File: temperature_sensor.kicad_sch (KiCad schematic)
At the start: 3 parts, among them U3 XIAO-SAMD21-SMD, U5 TMP37FT9Z

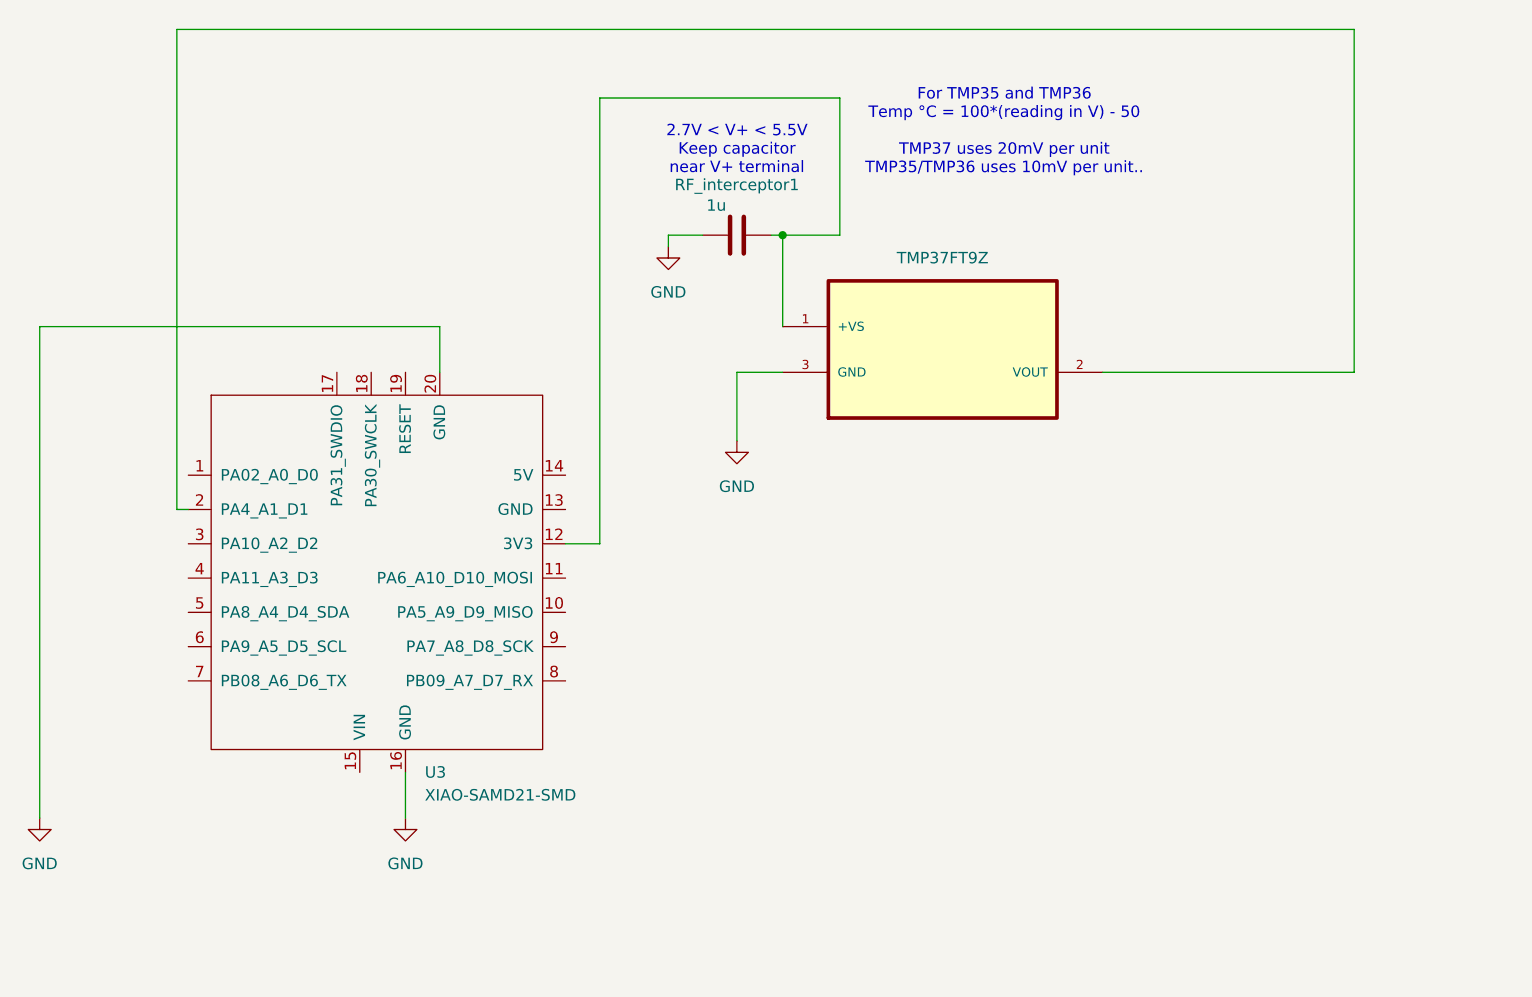
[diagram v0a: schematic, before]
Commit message: ok yeah no
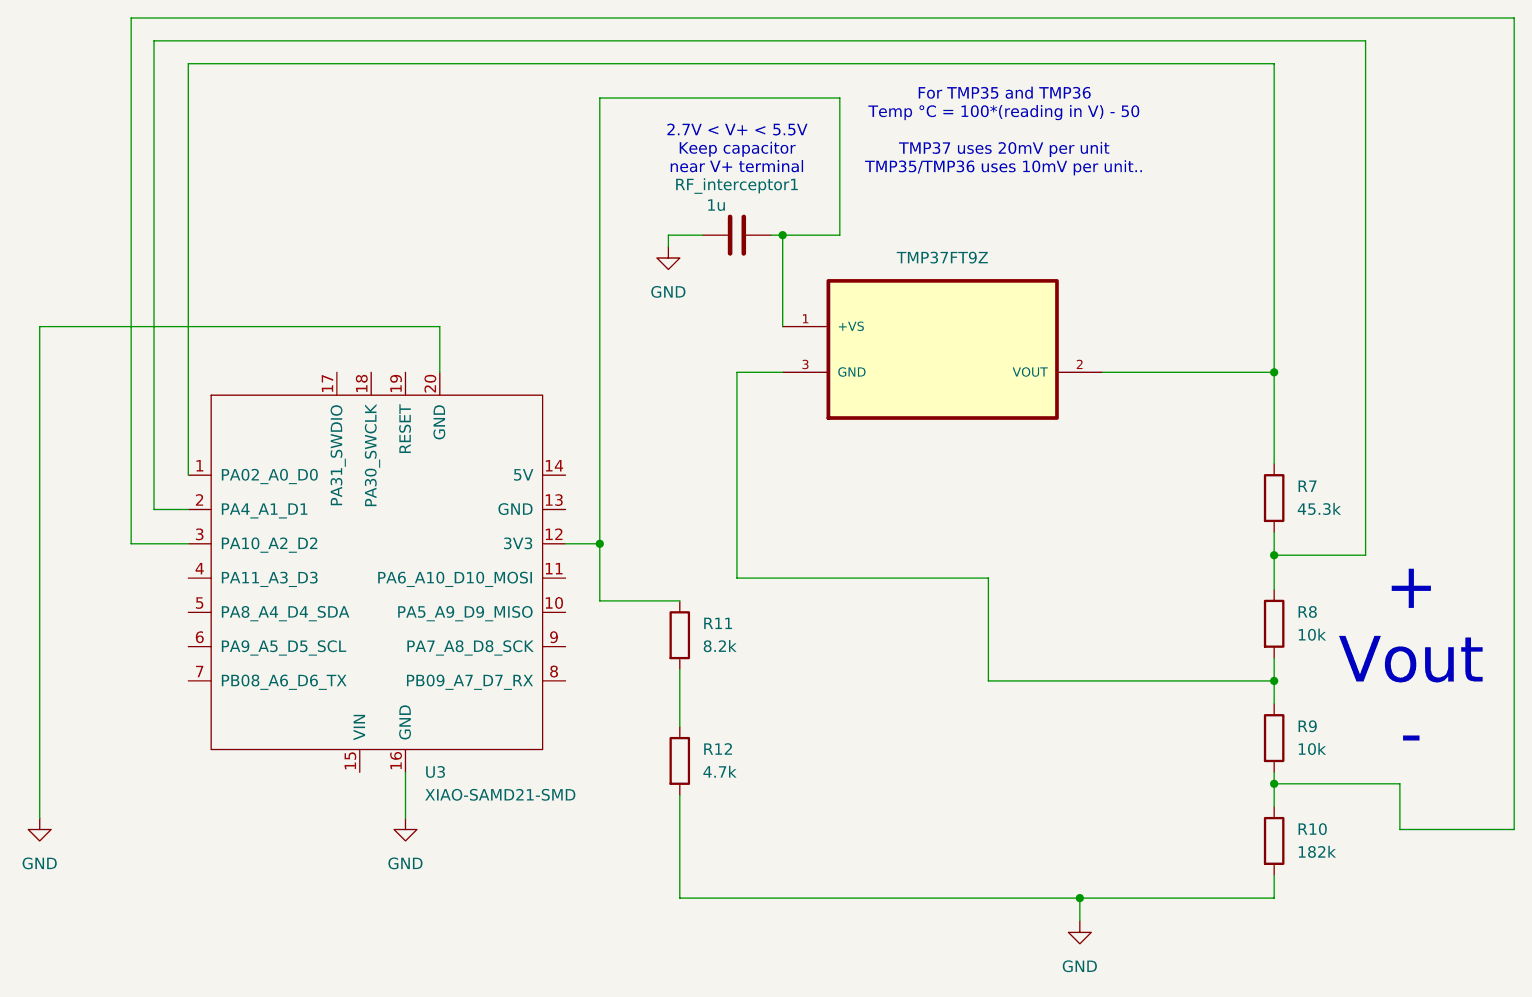
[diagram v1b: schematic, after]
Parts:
- added R10: 182k, Resistor_SMD:R_1210_3225Metric_Pad1.30x2.65mm_HandSolder, symbol Device:R
- added R11: 8.2k, R_1210_3225Metric_Pad1.30x2.65mm_HandSolder, symbol Device:R
- added R12: 4.7k, R_1210_3225Metric_Pad1.30x2.65mm_HandSolder, symbol Device:R
- added R7: 45.3k, R_1210_3225Metric_Pad1.30x2.65mm_HandSolder, symbol Device:R
- added R8, R9: 10k, R_1210_3225Metric_Pad1.30x2.65mm_HandSolder, symbol Device:R
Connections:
- net GND: now also R10.2, R12.2; no longer U5.3 (GND)
- net at RF_interceptor1.2, U3.12 (3V3), U5.1 (+VS): now also R11.1
- net at U5.2 (VOUT): now also U3.1 (PA02_A0_D0), R7.1; no longer U3.2 (PA4_A1_D1)
- net at U3.3 (PA10_A2_D2): now also R10.1, R9.2
- new net: R11.2, R12.1
- new net: R8.2, R9.1, U5.3 (GND)
- new net: R7.2, R8.1, U3.2 (PA4_A1_D1)
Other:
- note added: "+ Vout -"

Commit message: this is the one. simple and easy
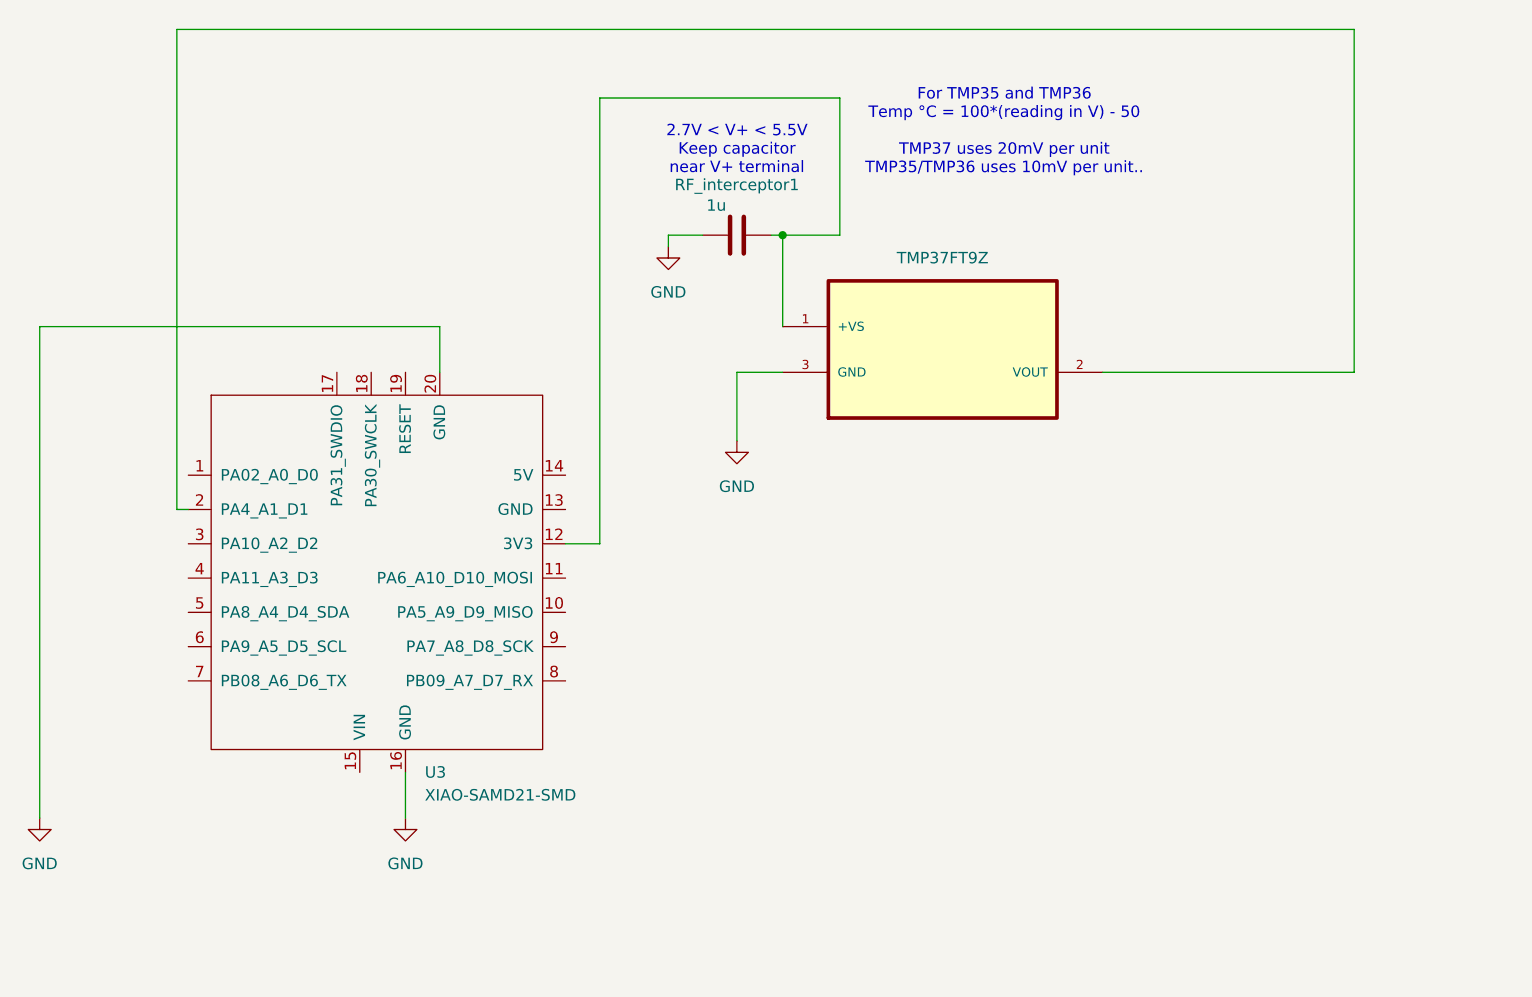
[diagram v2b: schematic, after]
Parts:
- removed R10: 182k, Resistor_SMD:R_1210_3225Metric_Pad1.30x2.65mm_HandSolder, symbol Device:R
- removed R11: 8.2k, R_1210_3225Metric_Pad1.30x2.65mm_HandSolder, symbol Device:R
- removed R12: 4.7k, R_1210_3225Metric_Pad1.30x2.65mm_HandSolder, symbol Device:R
- removed R7: 45.3k, R_1210_3225Metric_Pad1.30x2.65mm_HandSolder, symbol Device:R
- removed R8, R9: 10k, R_1210_3225Metric_Pad1.30x2.65mm_HandSolder, symbol Device:R
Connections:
- net GND: now also U5.3 (GND)
- net at U5.2 (VOUT): now also U3.2 (PA4_A1_D1); no longer U3.1 (PA02_A0_D0)
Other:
- note removed: "+ Vout -"
